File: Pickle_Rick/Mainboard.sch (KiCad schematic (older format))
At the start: 81 parts, among them J10 Conn_01x02_Male, J12 Conn_01x02_Male, J2 8P8C_LED, J3 Micro_SD_Card_Det, J9 Conn_01x02_Male, Q1 MMDT2222A, Q3 PMV20ENR, U1 CP2102N-A01-GQFN24, U10 PCA9536D, U2 SN65HVD230, U3 ESP32-WROOM-32D, U4 W25Q128JVSIM_TR, U5 MS5607-02BA

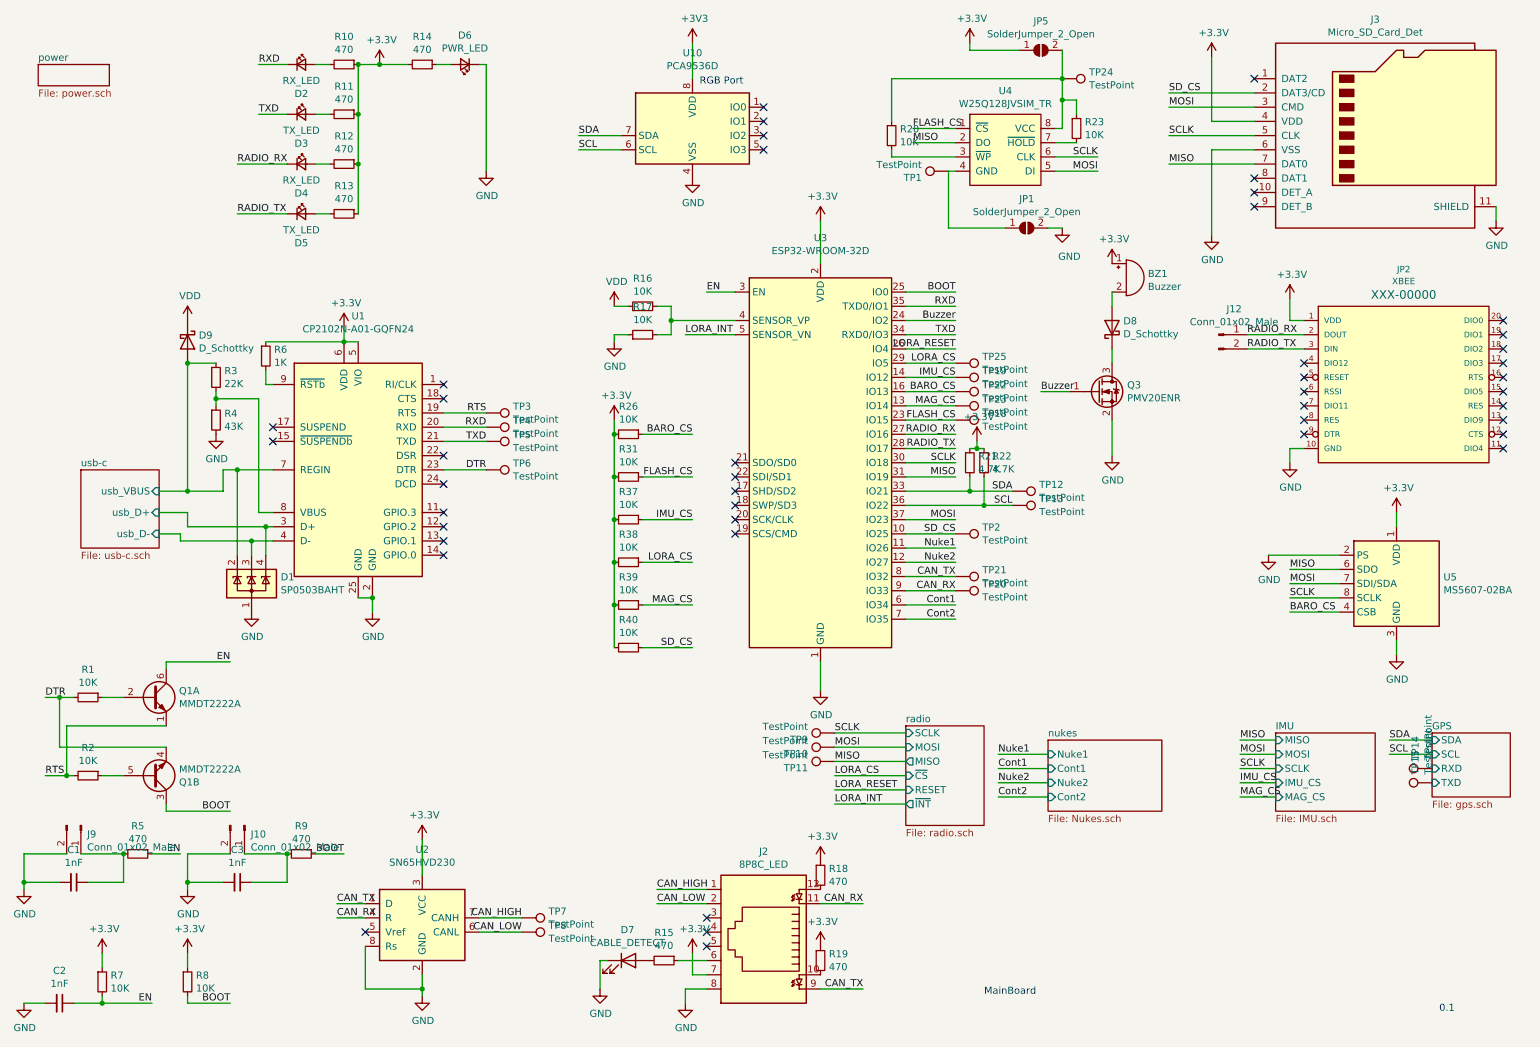
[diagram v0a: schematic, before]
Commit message: did some pcb thing
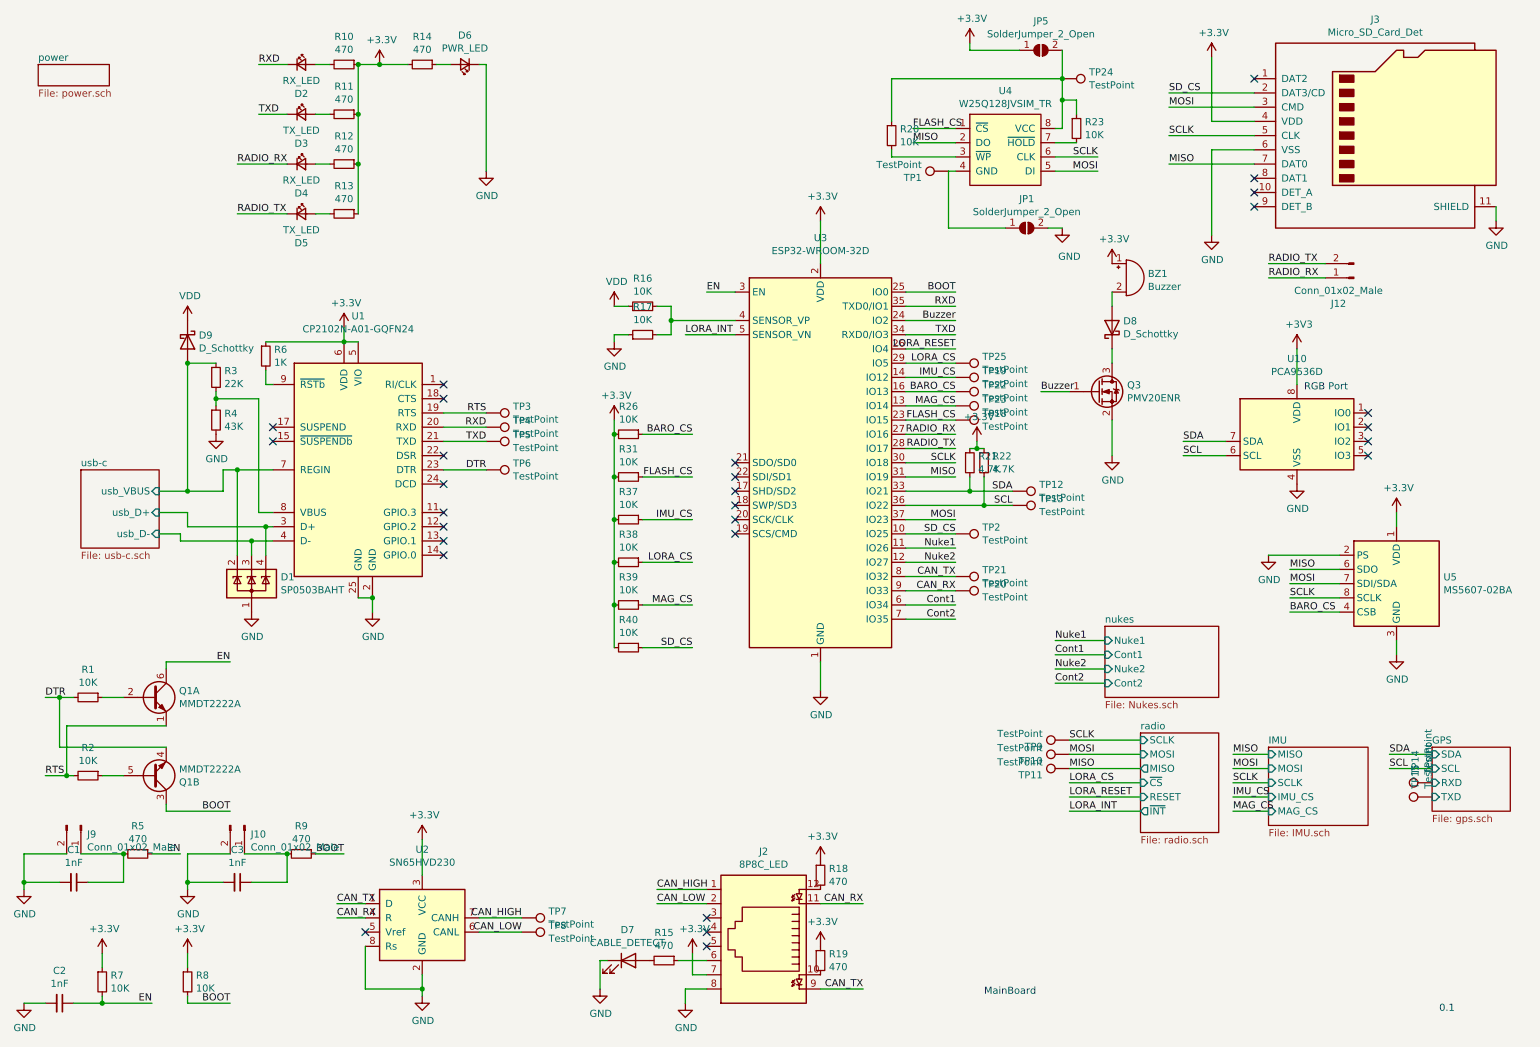
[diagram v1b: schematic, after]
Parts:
- removed JP2: XBEE, iclr:XBEE, symbol Mainboard-rescue:XBEE-iclr
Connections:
- no-connect marks 44 -> 28
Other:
- moved on the sheet: J12, TP10, TP11, TP14, TP15, TP9, U10
